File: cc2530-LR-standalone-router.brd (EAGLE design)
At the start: 44 x 24 mm, 16 parts, among them J1 629105150921, U1 AP2112K

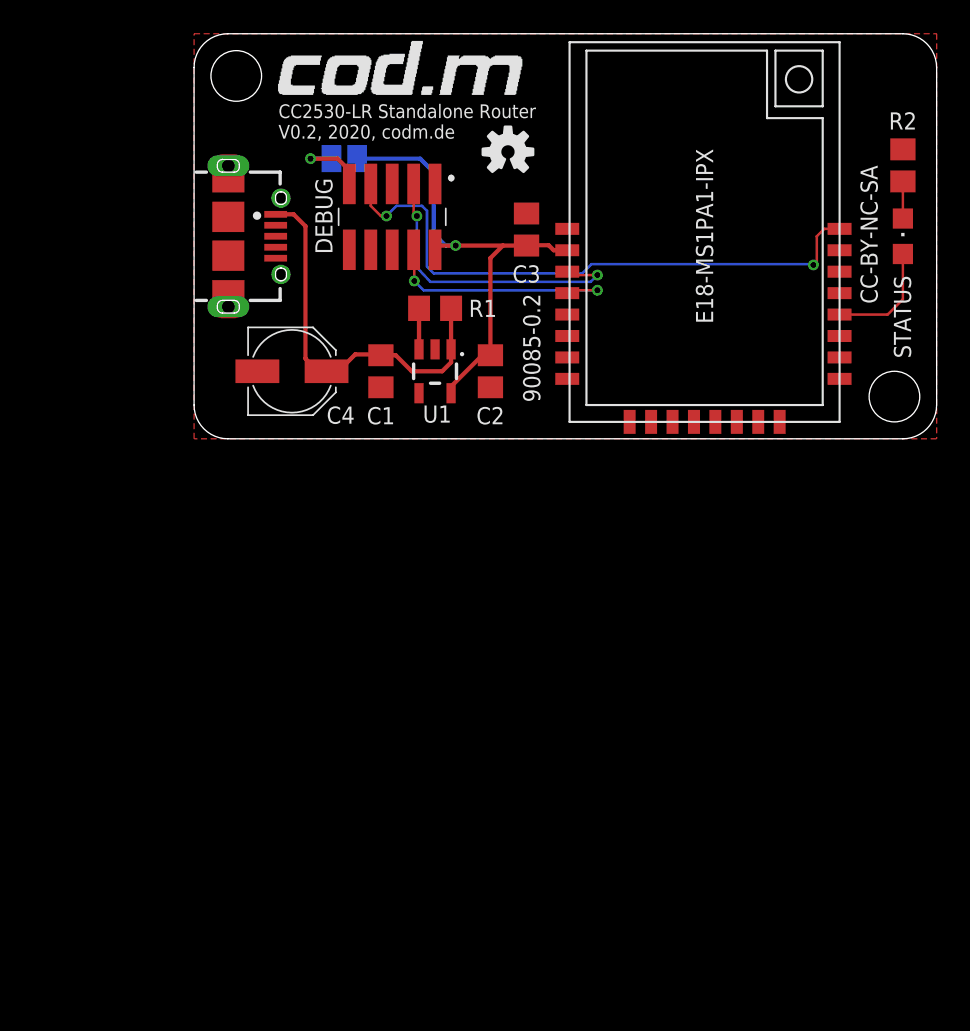
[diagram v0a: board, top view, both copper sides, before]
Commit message: Modified Version (USB Stick)
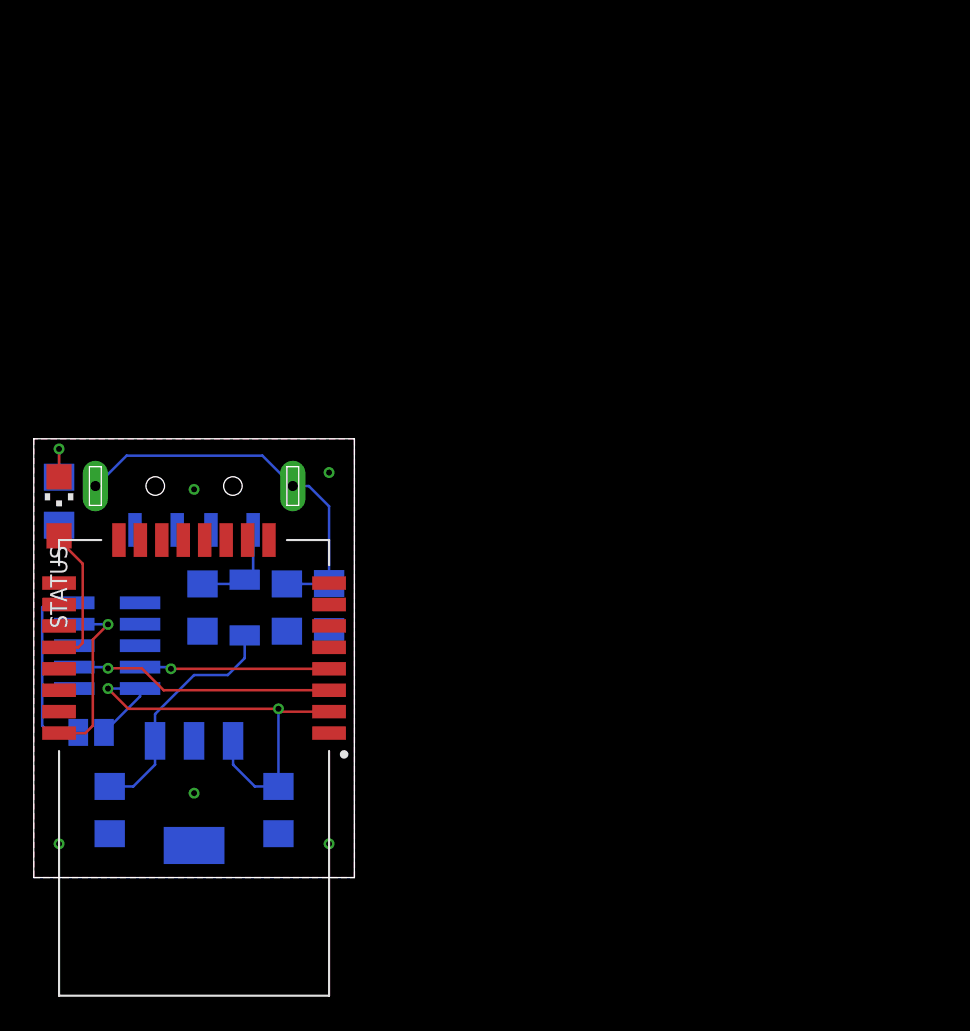
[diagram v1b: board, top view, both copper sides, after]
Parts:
- removed J1: 629105150921, WR-USB_Rev20b:629105150921
- removed U$1: (no value), codm:WEEE-LOGO-8MM
- removed U$2: (no value), codm:CODM-LOGO
- removed U$3: (no value), SparkFun-Aesthetics:OSHW-LOGO-M
- removed U$4: (no value), SparkFun-Aesthetics:OSHW-LOGO-S
- removed U1: AP2112K, SparkFun-IC-Power:SOT23-5
- added L1: 33n, inductor-neosid:SM-1206
- added U2: MCP1703-3302, dersimn_basics:SOT-22-3
- added X1: A-USB A-LP-SMT-C, dersimn_connector:A-USB_A-LP-SMT-C
- C1: value 1µ -> 4.7n; device rcl:C0805 -> rcl:C1206
- C2: value 1µ -> 10n; device rcl:C0805 -> rcl:C1206
- C3: value 100nF -> 1µF; device rcl:C0805 -> resistor:C1206
- C4: value 22u -> 1µF; device rcl:PANASONIC_C -> resistor:C1206
- R1: value 10k -> 1M; device rcl:R0805 -> rcl:R1206
- R2: device rcl:R0805 -> rcl:R1206
- STATUS: device led:CHIPLED_0805 -> led:CHIPLED_1206
- U$5: value E18-MS1PA1IPX -> E18-MS1PA2-PCB; device codm:E18-MS1PA1-IPX -> e18-ms1pa1-ipx:E18-MS1PA2-PCB
- moved R2 53.8 mm to (-8.00, -3.70), flipped to the bottom, turned to 90 degrees
- moved STATUS 52.5 mm to (-8.00, -4.00)
- moved C3 42.3 mm to (-5.00, -22.0), flipped to the bottom
- moved U$5 38.9 mm to (0.00, -6.00), turned to 270 degrees
- moved DBGVCC 37.2 mm to (-6.10, -17.4)
- moved DEBUG 30.5 mm to (-5.15, -12.3), flipped to the bottom, turned to 90 degrees
- moved C4 26.0 mm to (5.00, -22.0), flipped to the bottom, turned to 270 degrees
- moved C2 22.1 mm to (0.50, -10.0), flipped to the bottom, turned to 270 degrees
- moved R1 18.8 mm to (8.00, -10.0), flipped to the bottom, turned to 270 degrees
- moved C1 15.1 mm to (5.50, -10.0), flipped to the bottom, turned to 270 degrees
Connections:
- removed net N$1: R1.2, U1.3
- removed net VCC: C2.2, C3.2, DBGVCC.1, DEBUG.2, U$5.VCC, U1.5
- new net +3V3: C4.1, DBGVCC.1, DEBUG.2, U$5.2, U2.3
- new net SHIELD: C1.1, R1.1, X1.S1, X1.S2
- new net VUSB: C2.1, L1.1, X1.1
- net +5V: now also C3.1, L1.2, U2.1; no longer C1.2, C4.+, J1.1, R1.1, U1.1
- net DC: now also U$5.3; no longer U$5.P2.2
- net DD: now also U$5.4; no longer U$5.P2.1
- net GND: now also C1.2, C2.2, C3.2, C4.2, R1.2, U$5.1, U2.2, U2.4, X1.4; no longer C1.1, C2.1, C3.1, C4.-, J1.5, J1.S1, J1.S2, J1.S3, J1.S4, J1.S5, J1.S6, U$5.GND, U1.2
- net N$3: now also U$5.20; no longer U$5.P0.3
- net RST: now also U$5.24; no longer U$5.RST
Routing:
- net VCC: track 28.5 -> 0.00 mm, vias 1 -> 0
- net +3V3: track 0.00 -> 28.3 mm, vias 0 -> 2
- net RST: track 35.2 -> 10.6 mm, vias 2 -> 1
- net SHIELD: track 0.00 -> 22.9 mm
- net +5V: track 21.9 -> 14.3 mm
- net VCC-DEBUG: track 4.63 -> 11.3 mm, vias 1 -> 0
- net VUSB: track 0.00 -> 5.76 mm
- net DD: track 14.8 -> 11.2 mm, vias 2 -> 1
- net DC: track 18.1 -> 15.7 mm, vias 2 -> 1
- net N$1: track 2.43 -> 0.00 mm
- net N$3: track 6.81 -> 8.44 mm
- net N$2: track 2.20 -> 3.33 mm, vias 0 -> 1
- added copper zone on layer 16, net GND
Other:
- board size 44 x 24 mm -> 19 x 26 mm
- board text removed: "90085-0.2"
- board text removed: "90085-0.2 codm.de, 2020"
- board text removed: "CC-BY-NC-SA"
- board text removed: "CC2530-LR Standalone Router V0.2, 2020, codm.de"
